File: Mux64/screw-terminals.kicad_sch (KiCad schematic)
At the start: 111 parts, among them J11 Screw_Terminal_01x12, J12 Screw_Terminal_01x12, J13 Screw_Terminal_01x12, J14 Screw_Terminal_01x12, J15 Screw_Terminal_01x12, J16 Screw_Terminal_01x12, J17 Screw_Terminal_01x12, J18 Screw_Terminal_01x12

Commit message: Add files via upload
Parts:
- J11, J12, J13, J14, J15, J16, J17, J18: footprint (none) -> TerminalBlock_Phoenix:TerminalBlock_Phoenix_MPT-0,5-12-2.54_1x12_P2.54mm_Horizontal
- R10, R100, R101, R102, R103, R104, R105, R106, R107, R108, R109, R11, R110, R12, R13, R14, R15, R16, R17, R18, R19, R20, R21, R22, R23, R24, R25, R26, R27, R28, R29, R30, R31, R32, R39, R40, R41, R42, R43, R44, R45, R46, R47, R48, R49, R50, R57, R58, R59, R60, R61, R62, R63, R64, R65, R66, R67, R68, R69, R70, R71, R72, R73, R74, R75, R76, R77, R78, R79, R80, R81, R82, R83, R84, R85, R86, R87, R88, R89, R9, R90, R91, R92, R93, R94, R95, R96, R97, R98, R99: footprint (none) -> Resistor_SMD:R_0805_2012Metric
- R33, R34, R35, R36, R37, R38, R51, R52, R53, R54, R55, R56: footprint (none) -> Resistor_SMD:R_1206_3216Metric
- R8: footprint (none) -> Resistor_SMD:R_0603_1608Metric

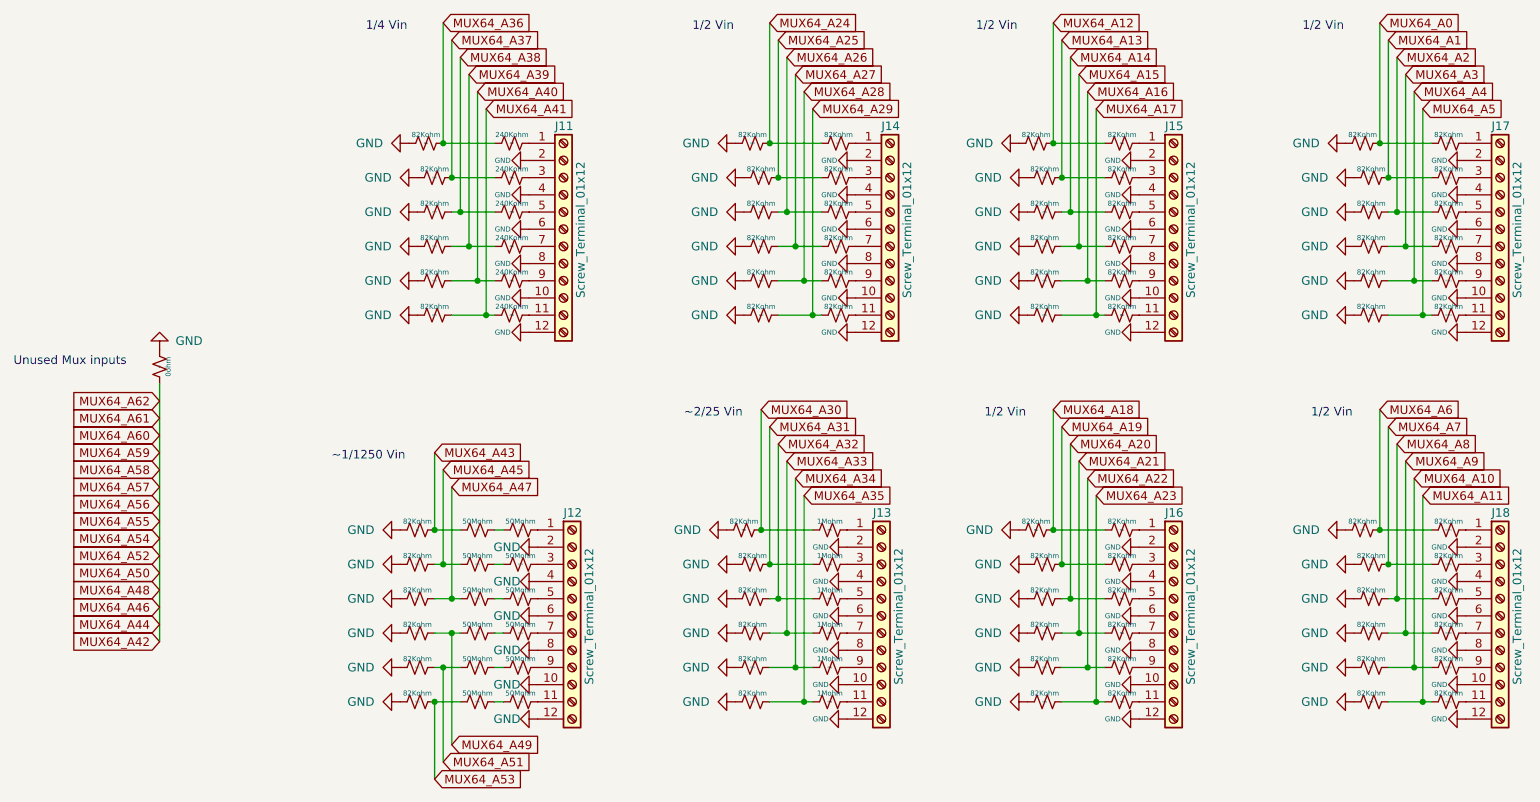
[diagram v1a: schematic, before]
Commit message: Add files via upload
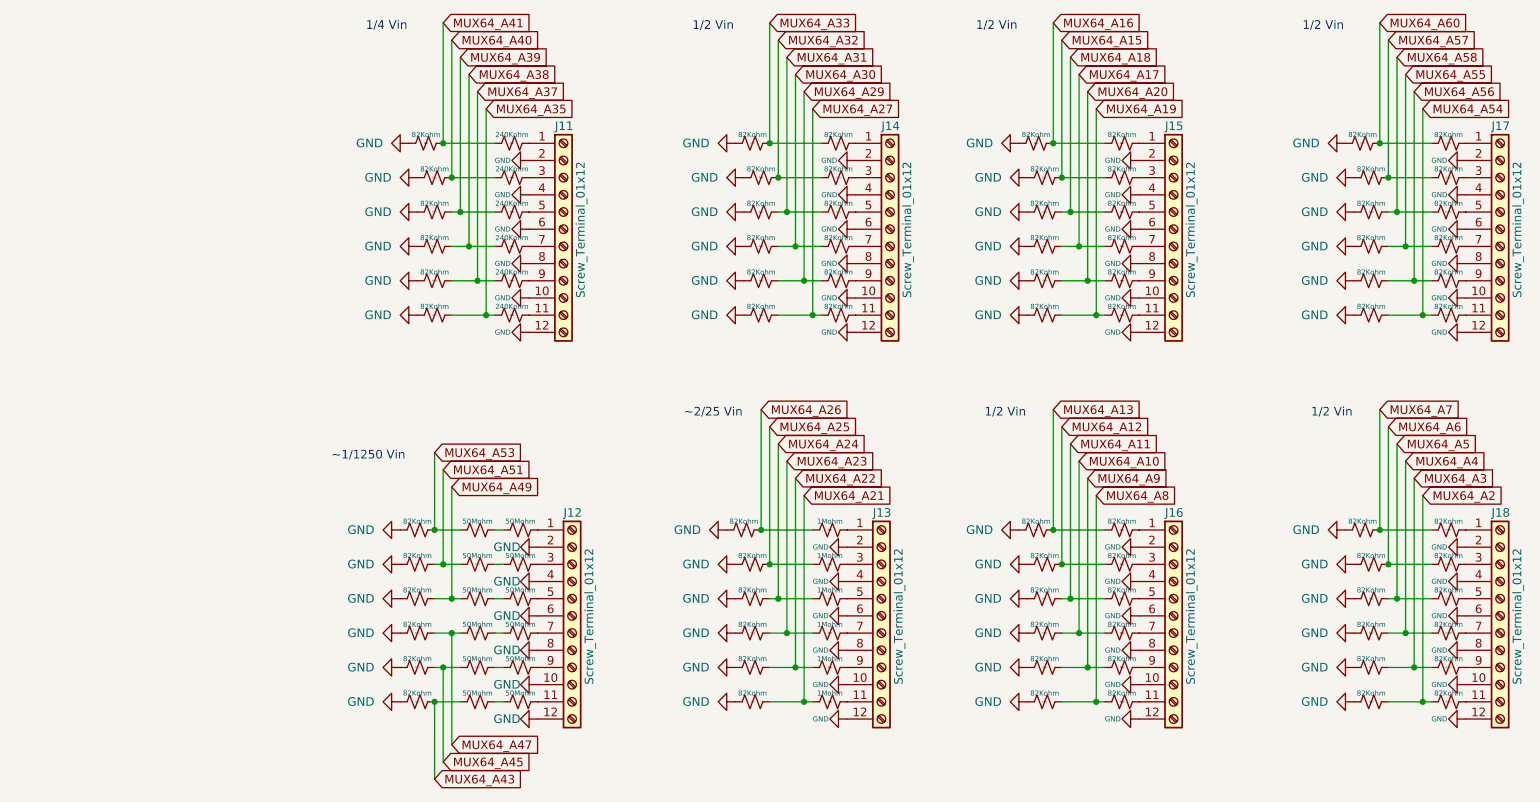
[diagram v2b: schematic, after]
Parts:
- removed R8: 0ohm, Resistor_SMD:R_0603_1608Metric, symbol Device:R_Small_US
- R21, R22, R23, R24, R25, R26: footprint Resistor_SMD:R_0805_2012Metric -> Resistor_SMD:R_1206_3216Metric
- R51, R52, R53, R54, R55, R56: footprint Resistor_SMD:R_1206_3216Metric -> Resistor_SMD:R_0805_2012Metric
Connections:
- net MUX64_A14 is gone; now on net MUX64_A18: R66.2, R77.1
- net MUX64_A28 is gone; now on net MUX64_A29: R49.2, R61.1
- net MUX64_A34 is gone; now on net MUX64_A22: R44.2, R55.1
- net MUX64_A36 is gone; now on net MUX64_A41: R15.2, R27.1
- net MUX64_A10: now also R72.2, R84.1; no longer R109.1, R97.2
- net MUX64_A11: now also R71.2, R83.1; no longer R110.1, R98.2
- net MUX64_A12: now also R70.2, R82.1; no longer R63.2, R75.1
- net MUX64_A13: now also R64.2, R81.1; no longer R65.2, R76.1
- net MUX64_A15: now also R65.2, R76.1; no longer R67.2, R78.1
- net MUX64_A16: now also R63.2, R75.1; no longer R68.2, R79.1
- net MUX64_A17: now also R67.2, R78.1; no longer R69.2, R80.1
- net MUX64_A18: no longer R64.2, R81.1
- net MUX64_A19: now also R69.2, R80.1; no longer R70.2, R82.1
- net MUX64_A2: now also R110.1, R98.2; no longer R101.1, R90.2
- net MUX64_A20: now also R68.2, R79.1; no longer R71.2, R83.1
- net MUX64_A21: now also R45.2, R56.1; no longer R72.2, R84.1
- net MUX64_A22: no longer R73.2, R85.1
- net MUX64_A23: now also R43.2, R54.1; no longer R74.2, R86.1
- net MUX64_A24: now also R42.2, R53.1; no longer R40.2, R57.1
- net MUX64_A25: now also R41.2, R52.1; no longer R46.2, R58.1
- net MUX64_A26: now also R39.2, R51.1; no longer R47.2, R59.1
- net MUX64_A27: now also R50.2, R62.1; no longer R48.2, R60.1
- net MUX64_A29: no longer R50.2, R62.1
- net MUX64_A3: now also R109.1, R97.2; no longer R102.1, R91.2
- net MUX64_A30: now also R48.2, R60.1; no longer R39.2, R51.1
- net MUX64_A31: now also R47.2, R59.1; no longer R41.2, R52.1
- net MUX64_A32: now also R46.2, R58.1; no longer R42.2, R53.1
- net MUX64_A33: now also R40.2, R57.1; no longer R43.2, R54.1
- net MUX64_A35: now also R20.2, R32.1; no longer R45.2, R56.1
- net MUX64_A37: now also R19.2, R31.1; no longer R16.2, R28.1
- net MUX64_A38: now also R18.2, R30.1; no longer R17.2, R29.1
- net MUX64_A39: now also R17.2, R29.1; no longer R18.2, R30.1
- net MUX64_A4: now also R108.1, R96.2; no longer R103.1, R92.2
- net MUX64_A40: now also R16.2, R28.1; no longer R19.2, R31.1
- net MUX64_A41: no longer R20.2, R32.1
- net MUX64_A43: now also R14.2, R26.1; no longer R21.1, R9.2
- net MUX64_A45: now also R13.2, R25.1; no longer R10.2, R22.1
- net MUX64_A47: now also R12.2, R24.1; no longer R11.2, R23.1
- net MUX64_A49: now also R11.2, R23.1; no longer R12.2, R24.1
- net MUX64_A5: now also R107.1, R95.2; no longer R104.1, R93.2
- net MUX64_A51: now also R10.2, R22.1; no longer R13.2, R25.1
- net MUX64_A53: now also R21.1, R9.2; no longer R14.2, R26.1
- net MUX64_A6: now also R106.1, R94.2; no longer R105.1, R88.2
- net MUX64_A7: now also R105.1, R88.2; no longer R106.1, R94.2
- net MUX64_A8: now also R74.2, R86.1; no longer R107.1, R95.2
- net MUX64_A9: now also R73.2, R85.1; no longer R108.1, R96.2
- net MUX64_A0 renamed MUX64_A60
- net MUX64_A1 renamed MUX64_A57
- new net MUX64_A54: R104.1, R93.2
- new net MUX64_A55: R102.1, R91.2
- new net MUX64_A56: R103.1, R92.2
- new net MUX64_A58: R101.1, R90.2
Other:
- note removed: "Unused Mux inputs"
